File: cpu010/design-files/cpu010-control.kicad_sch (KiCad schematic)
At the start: 26 parts, among them SW401 SW_DIP_x08, SW402 SW_DIP_x08, U401 DA04-11SURKWA, U402 74HCT273, U403 74HCT273, U404 GAL22V10, U405 74HC245, U406 74HC245, U407 74HCT273, U408 74HC245, U409 ATF1504AS-PLCC44

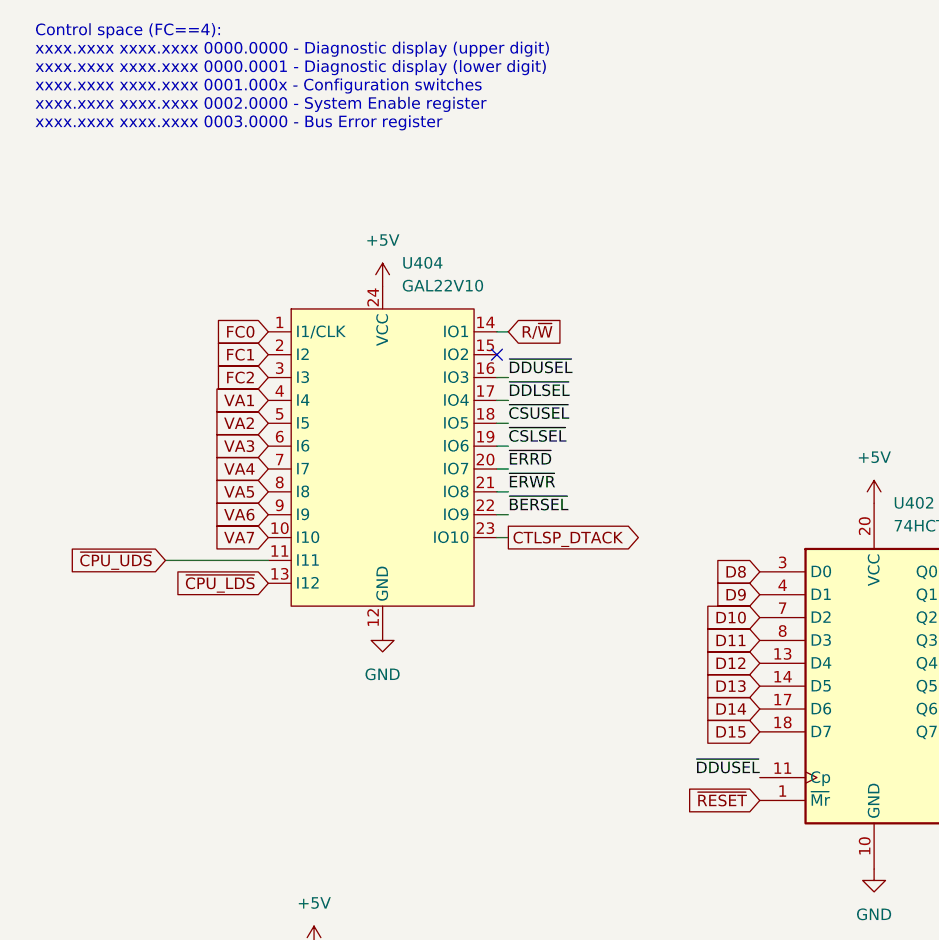
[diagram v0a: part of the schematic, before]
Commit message: Document IOCTL address decode.
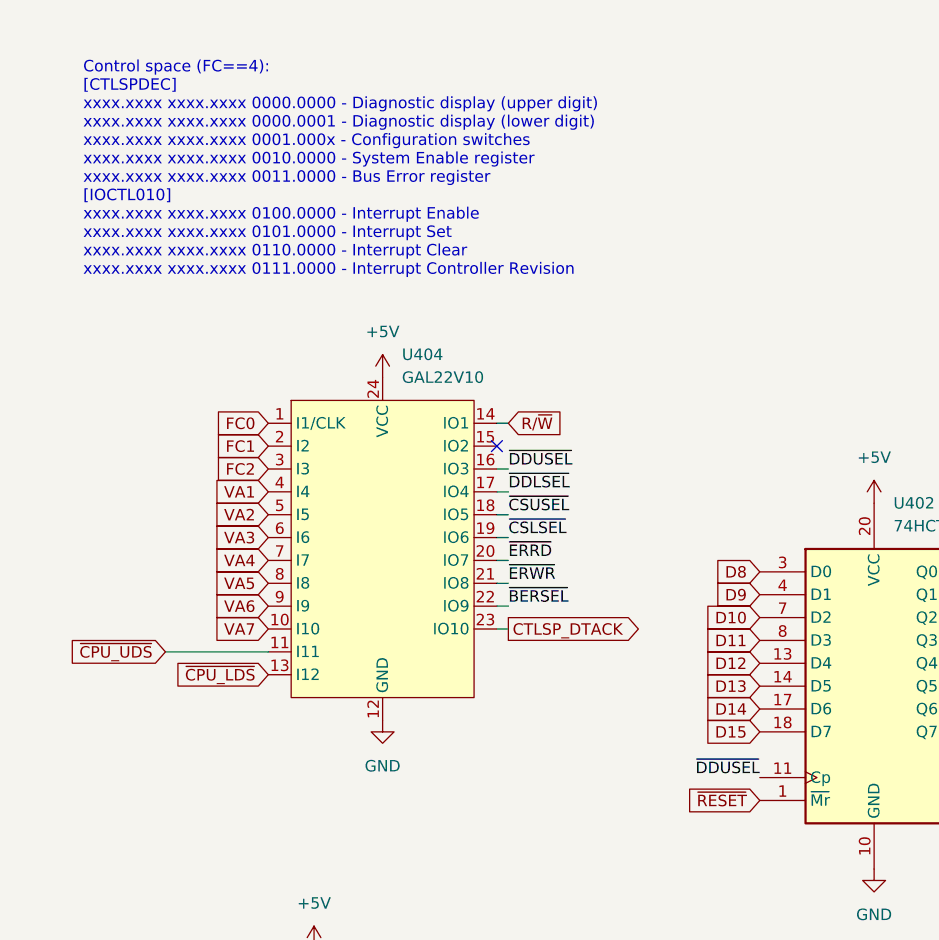
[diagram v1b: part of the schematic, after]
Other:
- note added: "Control space (FC==4): [CTLSPDEC] xxxx.xxxx xxxx.xxxx 0000.0000 - Diagnostic display (upper digit) xxxx.xxxx xxxx.xxxx 0000.0001 - Diagnostic display (lower digit) xxxx.xxxx xxxx.xxxx 0001.000x - Configuration switches xxxx.xxxx xxxx.xxxx 0010.0000 - System Enable register xxxx.xxxx xxxx.xxxx 0011.0000 - Bus Error register [IOCTL010] xxxx.xxxx xxxx.xxxx 0100.0000 - Interrupt Enable xxxx.xxxx xxxx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"
- note removed: "Control space (FC==4): xxxx.xxxx xxxx.xxxx 0000.0000 - Diagnostic display (upper digit) xxxx.xxxx xxxx.xxxx 0000.0001 - Diagnostic display (lower digit) xxxx.xxxx xxxx.xxxx 0001.000x - Configuration switches xxxx.xxxx xxxx.xxxx 0002.0000 - System Enable register xxxx.xxxx xxxx.xxxx 0003.0000 - Bus Error register"
- moved on the sheet: U404
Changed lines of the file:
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@@
 	(generator_version "9.0")
 	(paper "A3")
-	(text "Control space (FC==4):\nxxxx.xxxx xxxx.xxxx 0000.0000 - Diagnostic display (upper digit)\nxxxx.xxxx xxxx.xxxx 0000.0001 - Diagnostic display (lower digit)\nxxxx.xxxx xxxx.xxxx 0001.000x - Configuration switches\nxxxx.xxxx xxxx.xxxx 0002.0000 - System Enable register\nxxxx.xxxx xxxx.xxxx 0003.0000 - Bus Error register"
+	(text "Control space (FC==4):\n[CTLSPDEC]\nxxxx.xxxx xxxx.xxxx 0000.0000 - Diagnostic display (upper digit)\nxxxx.xxxx xxxx.xxxx 0000.0001 - Diagnostic display (lower digit)\nxxxx.xxxx xxxx.xxxx 0001.000x - Configuration switches\nxxxx.xxxx xxxx.xxxx 0010.0000 - System Enable register\nxxxx.xxxx xxxx.xxxx 0011.0000 - Bus Error register\n[IOCTL010]\nxxxx.xxxx xxxx.xxxx 0100.0000 - Interrupt Enable\nxxxx.xxxx xxxx.xxxx 0101.0000 - Interrupt Set\nxxxx.xxxx xxxx.xxxx 0110.0000 - Interrupt Clear\nxxxx.xxxx xxxx.xxxx 0111.0000 - Interrupt Controller Revision"
 		(exclude_from_sim no)
-		(at 16.002 20.066 0)
+		(at 21.336 30.226 0)
 		(effects
 			(font
@@
 	)
 	(no_connect
-		(at 67.31 50.8)
+		(at 67.31 60.96)
 	)
 	(no_connect
@@
 	(wire
 		(pts
-			(xy 68.58 60.96) (xy 67.31 60.96)
+			(xy 68.58 71.12) (xy 67.31 71.12)
 		)
 		(stroke
@@
 	(wire
 		(pts
-			(xy 67.31 68.58) (xy 68.58 68.58)
+			(xy 67.31 78.74) (xy 68.58 78.74)
 		)
 		(stroke
@@
 	(wire
 		(pts
-			(xy 68.58 66.04) (xy 67.31 66.04)
+			(xy 68.58 76.2) (xy 67.31 76.2)
 		)
 		(stroke
@@
 	(wire
 		(pts
-			(xy 68.58 58.42) (xy 67.31 58.42)
+			(xy 68.58 68.58) (xy 67.31 68.58)
 		)
 		(stroke
@@
 	(wire
 		(pts
-			(xy 68.58 48.26) (xy 67.31 48.26)
+			(xy 68.58 58.42) (xy 67.31 58.42)
 		)
 		(stroke
@@
 	(wire
 		(pts
-			(xy 30.48 73.66) (xy 41.91 73.66)
+			(xy 30.48 83.82) (xy 41.91 83.82)
 		)
 		(stroke
@@
 	(wire
 		(pts
-			(xy 68.58 55.88) (xy 67.31 55.88)
+			(xy 68.58 66.04) (xy 67.31 66.04)
 		)
 		(stroke
@@
 	(wire
 		(pts
-			(xy 68.58 71.12) (xy 67.31 71.12)
+			(xy 68.58 81.28) (xy 67.31 81.28)
 		)
 		(stroke
@@
 	(wire
 		(pts
-			(xy 68.58 63.5) (xy 67.31 63.5)
+			(xy 68.58 73.66) (xy 67.31 73.66)
 		)
 		(stroke
@@
 	(wire
 		(pts
-			(xy 68.58 53.34) (xy 67.31 53.34)
+			(xy 68.58 63.5) (xy 67.31 63.5)
 		)
 		(stroke
@@
 	)
 	(label "~{CSLSEL}"
-		(at 68.58 60.96 0)
+		(at 68.58 71.12 0)
 		(effects
 			(font
@@
 	)
 	(label "~{CSUSEL}"
-		(at 68.58 58.42 0)
+		(at 68.58 68.58 0)
 		(effects
 			(font
@@
 	)
 	(label "~{BERSEL}"
-		(at 68.58 68.58 0)
+		(at 68.58 78.74 0)
 		(effects
 			(font
@@
 	)
 	(label "~{DDLSEL}"
-		(at 68.58 55.88 0)
+		(at 68.58 66.04 0)
 		(effects
 			(font
@@
 	)
 	(label "~{ERWR}"
-		(at 68.58 66.04 0)
+		(at 68.58 76.2 0)
 		(effects
 			(font
@@
 	)
 	(label "~{DDUSEL}"
-		(at 68.58 53.34 0)
+		(at 68.58 63.5 0)
 		(effects
 			(font
@@
 	)
 	(label "~{ERRD}"
-		(at 68.58 63.5 0)
+		(at 68.58 73.66 0)
 		(effects
 			(font
@@
 	(global_label "R{slash}~{W}"
 		(shape input)
-		(at 68.58 48.26 0)
+		(at 68.58 58.42 0)
 		(fields_autoplaced yes)
 		(effects
@@
 		)
 		(property "Intersheetrefs" "${INTERSHEET_REFS}"
-			(at 75.6171 48.26 0)
+			(at 75.6171 58.42 0)
 			(effects
 				(font
@@
 	(global_label "VA1"
 		(shape input)
-		(at 41.91 55.88 180)
+		(at 41.91 66.04 180)
 		(fields_autoplaced yes)
 		(effects
@@
 		)
 		(property "Intersheetrefs" "${INTERSHEET_REFS}"
-			(at 35.5381 55.88 0)
+			(at 35.5381 66.04 0)
 			(effects
 				(font
@@
 	(global_label "FC0"
 		(shape input)
-		(at 41.91 48.26 180)
+		(at 41.91 58.42 180)
 		(fields_autoplaced yes)
 		(effects
@@
 		)
 		(property "Intersheetrefs" "${INTERSHEET_REFS}"
-			(at 35.3567 48.26 0)
+			(at 35.3567 58.42 0)
 			(effects
 				(font
@@
 	(global_label "~{CPU_UDS}"
 		(shape input)
-		(at 30.48 73.66 180)
+		(at 30.48 83.82 180)
 		(fields_autoplaced yes)
 		(effects
@@
 		)
 		(property "Intersheetrefs" "${INTERSHEET_REFS}"
-			(at 18.8467 73.66 0)
+			(at 18.8467 83.82 0)
 			(effects
 				(font
@@
 	(global_label "VA2"
 		(shape input)
-		(at 41.91 58.42 180)
+		(at 41.91 68.58 180)
 		(fields_autoplaced yes)
 		(effects
@@
 		)
 		(property "Intersheetrefs" "${INTERSHEET_REFS}"
-			(at 35.5381 58.42 0)
+			(at 35.5381 68.58 0)
 			(effects
 				(font
@@
 	(global_label "FC2"
 		(shape input)
-		(at 41.91 53.34 180)
+		(at 41.91 63.5 180)
 		(fields_autoplaced yes)
 		(effects
@@
 		)
 		(property "Intersheetrefs" "${INTERSHEET_REFS}"
-			(at 35.3567 53.34 0)
+			(at 35.3567 63.5 0)
 			(effects
 				(font
@@
 	(global_label "FC1"
 		(shape input)
-		(at 41.91 50.8 180)
+		(at 41.91 60.96 180)
 		(fields_autoplaced yes)
 		(effects
@@
 		)
 		(property "Intersheetrefs" "${INTERSHEET_REFS}"
-			(at 35.3567 50.8 0)
+			(at 35.3567 60.96 0)
 			(effects
 				(font
@@
 	(global_label "VA7"
 		(shape input)
-		(at 41.91 71.12 180)
+		(at 41.91 81.28 180)
 		(fields_autoplaced yes)
 		(effects
@@
 		)
 		(property "Intersheetrefs" "${INTERSHEET_REFS}"
-			(at 35.5381 71.12 0)
+			(at 35.5381 81.28 0)
 			(effects
 				(font
@@
 	(global_label "~{CPU_LDS}"
 		(shape input)
-		(at 41.91 76.2 180)
+		(at 41.91 86.36 180)
 		(fields_autoplaced yes)
 		(effects
@@
 		)
 		(property "Intersheetrefs" "${INTERSHEET_REFS}"
-			(at 30.5791 76.2 0)
+			(at 30.5791 86.36 0)
 			(effects
 				(font
@@
 	(global_label "VA3"
 		(shape input)
-		(at 41.91 60.96 180)
+		(at 41.91 71.12 180)
 		(fields_autoplaced yes)
 		(effects
@@
 		)
 		(property "Intersheetrefs" "${INTERSHEET_REFS}"
-			(at 35.5381 60.96 0)
+			(at 35.5381 71.12 0)
 			(effects
 				(font
@@
 	(global_label "VA6"
 		(shape input)
-		(at 41.91 68.58 180)
+		(at 41.91 78.74 180)
 		(fields_autoplaced yes)
 		(effects
@@
 		)
 		(property "Intersheetrefs" "${INTERSHEET_REFS}"
-			(at 35.5381 68.58 0)
+			(at 35.5381 78.74 0)
 			(effects
 				(font
@@
 	(global_label "CTLSP_DTACK"
 		(shape output)
-		(at 68.58 71.12 0)
+		(at 68.58 81.28 0)
 		(fields_autoplaced yes)
 		(effects
@@
 		)
 		(property "Intersheetrefs" "${INTERSHEET_REFS}"
-			(at 84.1442 71.12 0)
+			(at 84.1442 81.28 0)
 			(effects
 				(font
@@
 	(global_label "VA4"
 		(shape input)
-		(at 41.91 63.5 180)
+		(at 41.91 73.66 180)
 		(fields_autoplaced yes)
 		(effects
@@
 		)
 		(property "Intersheetrefs" "${INTERSHEET_REFS}"
-			(at 35.5381 63.5 0)
+			(at 35.5381 73.66 0)
 			(effects
 				(font
@@
 	(global_label "VA5"
 		(shape input)
-		(at 41.91 66.04 180)
+		(at 41.91 76.2 180)
 		(fields_autoplaced yes)
 		(effects
@@
 		)
 		(property "Intersheetrefs" "${INTERSHEET_REFS}"
-			(at 35.5381 66.04 0)
+			(at 35.5381 76.2 0)
 			(effects
 				(font
@@
 	(symbol
 		(lib_id "jrt-ICs:GAL22V10")
-		(at 54.61 62.23 0)
+		(at 54.61 72.39 0)
 		(unit 1)
 		(exclude_from_sim no)
@@
 		(fields_autoplaced yes)
 		(property "Reference" "U404"
-			(at 56.7533 40.64 0)
+			(at 56.7533 50.8 0)
 			(effects
 				(font
@@
 		)
 		(property "Value" "GAL22V10"
-			(at 56.7533 43.18 0)
+			(at 56.7533 53.34 0)
 			(effects
 				(font
@@
 		)
 		(property "Footprint" "Package_DIP:DIP-24_W7.62mm_Socket"
-			(at 54.61 62.23 0)
+			(at 54.61 72.39 0)
 			(effects
 				(font
@@
 		)
 		(property "Datasheet" ""
-			(at 54.61 62.23 0)
+			(at 54.61 72.39 0)
 			(effects
 				(font
@@
 		)
 		(property "Description" ""
-			(at 54.61 62.23 0)
+			(at 54.61 72.39 0)
 			(effects
 				(font
@@
 	(symbol
 		(lib_id "power:GND")
-		(at 54.61 81.28 0)
+		(at 54.61 91.44 0)
 		(unit 1)
 		(exclude_from_sim no)
@@
 		(fields_autoplaced yes)
 		(property "Reference" "#PWR0407"
-			(at 54.61 87.63 0)
+			(at 54.61 97.79 0)
 			(effects
 				(font
@@
 		)
 		(property "Value" "GND"
-			(at 54.61 86.36 0)
+			(at 54.61 96.52 0)
 			(effects
 				(font
@@
 		)
 		(property "Footprint" ""
-			(at 54.61 81.28 0)
+			(at 54.61 91.44 0)
 			(effects
 				(font
@@
 		)
 		(property "Datasheet" ""
-			(at 54.61 81.28 0)
+			(at 54.61 91.44 0)
 			(effects
 				(font
@@
 		)
 		(property "Description" "Power symbol creates a global label with name \"GND\" , ground"
-			(at 54.61 81.28 0)
+			(at 54.61 91.44 0)
 			(effects
 				(font
@@
 	(symbol
 		(lib_id "power:+5V")
-		(at 54.61 43.18 0)
+		(at 54.61 53.34 0)
 		(unit 1)
 		(exclude_from_sim no)
@@
 		(fields_autoplaced yes)
 		(property "Reference" "#PWR0406"
-			(at 54.61 46.99 0)
+			(at 54.61 57.15 0)
 			(effects
 				(font
@@
 		)
 		(property "Value" "+5V"
-			(at 54.61 38.1 0)
+			(at 54.61 48.26 0)
 			(effects
 				(font
@@
 		)
 		(property "Footprint" ""
-			(at 54.61 43.18 0)
+			(at 54.61 53.34 0)
 			(effects
 				(font
@@
 		)
 		(property "Datasheet" ""
-			(at 54.61 43.18 0)
+			(at 54.61 53.34 0)
 			(effects
 				(font
@@
 		)
 		(property "Description" "Power symbol creates a global label with name \"+5V\""
-			(at 54.61 43.18 0)
+			(at 54.61 53.34 0)
 			(effects
 				(font
